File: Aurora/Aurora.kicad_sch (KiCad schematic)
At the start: 44 parts, among them J1 UJ20-C-H-C-3-SMT-TR, U1 STM32H757BITx, U2 USBLC6-2SC6, U3 TLV76733DRVx, U4 AP63205WU-7

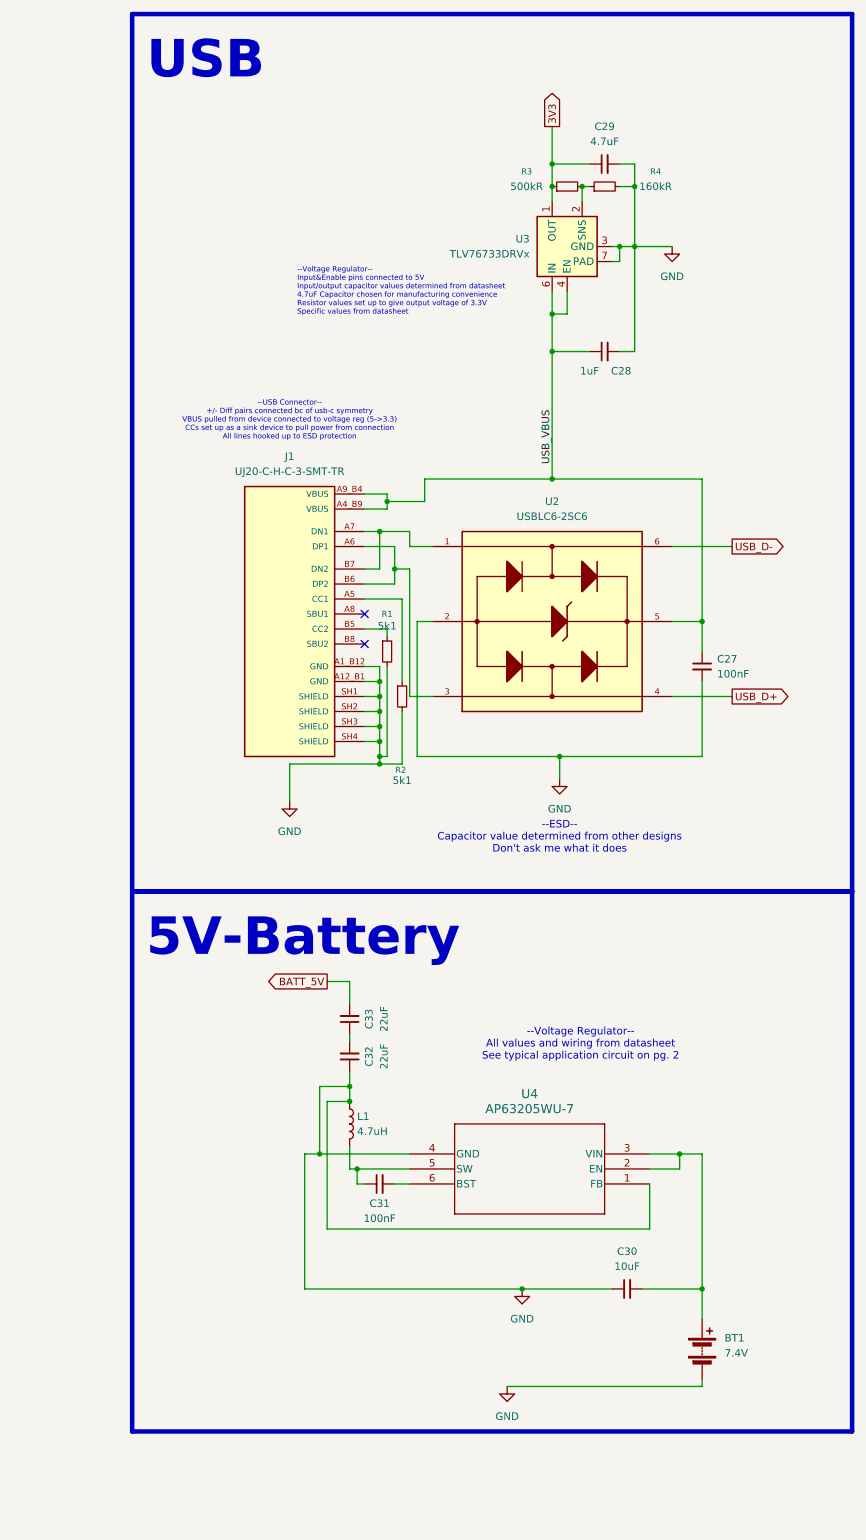
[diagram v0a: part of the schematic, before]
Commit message: power multiplexer
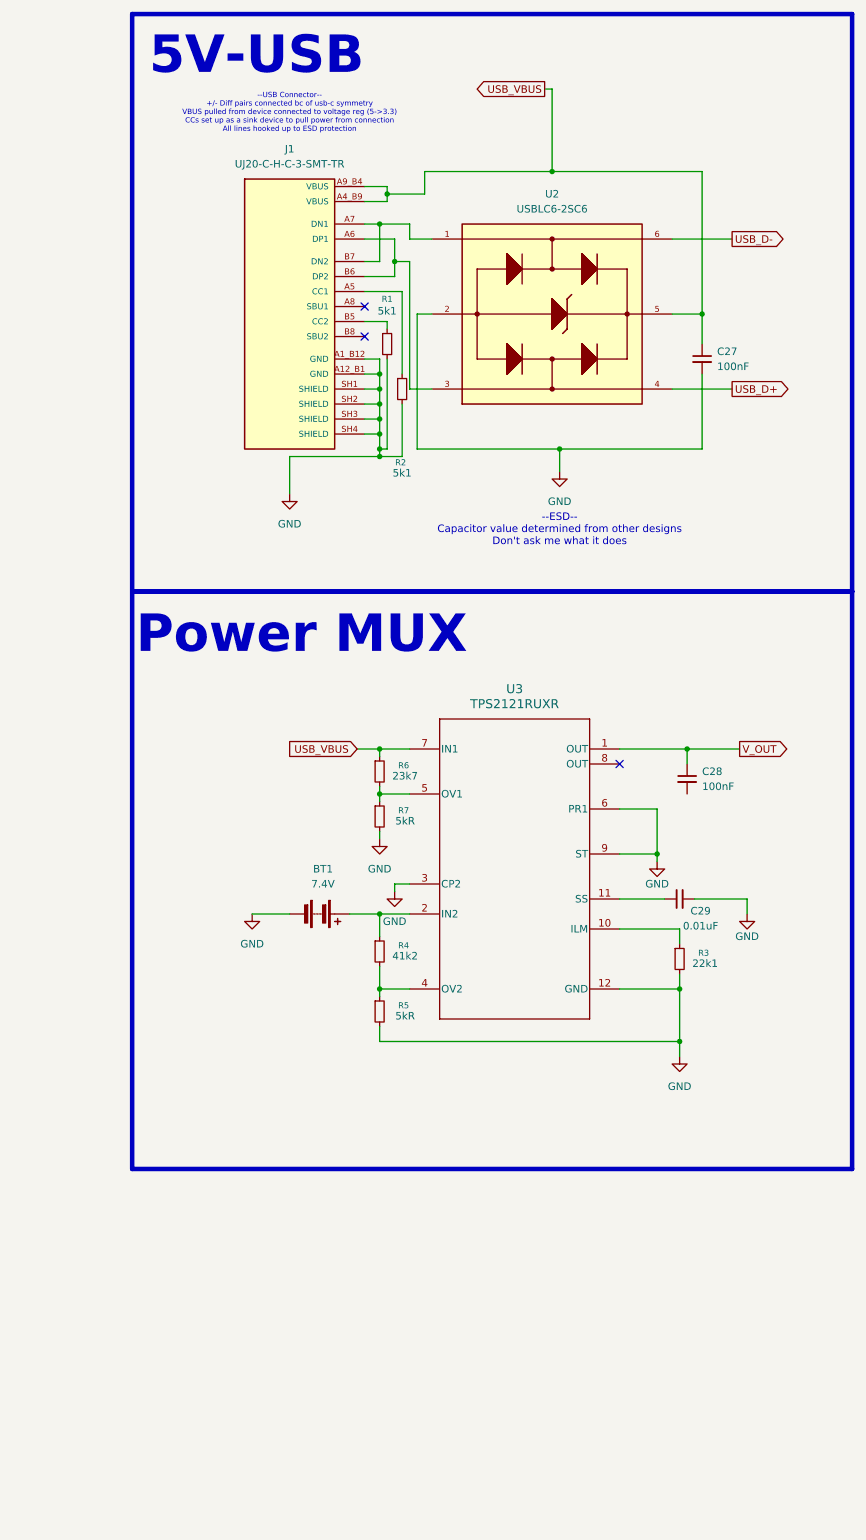
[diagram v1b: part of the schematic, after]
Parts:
- removed C30: 10uF, symbol Device:C_Small
- removed C31: 100nF, symbol Device:C_Small
- removed C32, C33: 22uF, symbol Device:C_Small
- removed L1: 4.7uH, symbol Device:L
- removed U3: TLV76733DRVx, Package_SON:WSON-6-1EP_2x2mm_P0.65mm_EP1x1.6mm_ThermalVias, symbol Regulator_Linear:TLV76733DRVx
- removed U4: AP63205WU-7, SOIC_05WU-7_DIO, symbol 2025-09-13_17-48-58:AP63205WU-7
- added R5, R7: 5kR, symbol Device:R_Small
- added R6: 23k7, symbol Device:R_Small
- added U3: TPS2121RUXR, footprints1:RUX0012A, symbol 2025-09-13_19-11-07:TPS2121RUXR
- C28: value 1uF -> 100nF
- C29: value 4.7uF -> 0.01uF
- R3: value 500kR -> 22k1
- R4: value 160kR -> 41k2
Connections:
- net 3V3: no longer C29.1, R3.1
- net GND: now also R3.2, R5.2, R7.2, U3.12 (GND), U3.3 (CP2), U3.6 (PR1), U3.9 (ST); no longer C28.2, R4.2
- net USB_VBUS: now also R6.1, U3.7 (IN1); no longer C28.1
- net at BT1.1 (+): now also R4.1, U3.2 (IN2)
- new net: R3.1, U3.10 (ILM)
- new net: C29.1, U3.11 (SS)
- new net: R4.2, R5.1, U3.4 (OV2)
- new net: R6.2, R7.1, U3.5 (OV1)
- new net V_OUT: C28.1, U3.1 (OUT)
- no-connect marks 2 -> 3
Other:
- note added: "5V-USB"
- note added: "Power MUX"
- note removed: "--Voltage Regulator-- All values and wiring from datasheet See typical application circuit on pg. 2"
- note removed: "--Voltage Regulator-- Input&Enable pins connected to 5V Input/output capacitor values determined from datasheet 4.7uF Capacitor chosen for manufacturing convenience Resistor values set up to give output voltage of 3.3V Specific values from datasheet"
- note removed: "5V-Battery"
- note removed: "USB"
- moved on the sheet: C27, J1, R1, R2, U2
